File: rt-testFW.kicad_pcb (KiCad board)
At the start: 2 copper layers, 11 parts, among them J1 1Min, J2 2Min, J3 3Min, J4 5Min, SW1 TestStart-Peach, SW2 Reset-Black

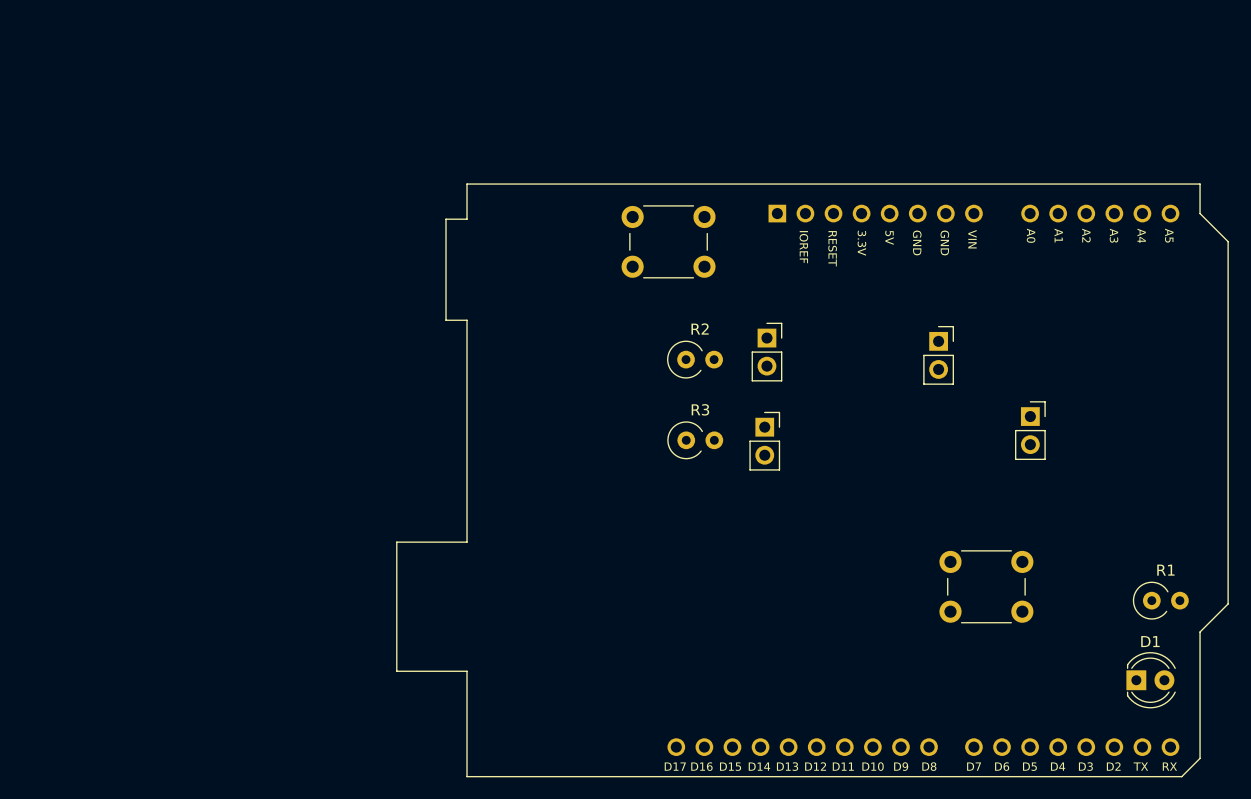
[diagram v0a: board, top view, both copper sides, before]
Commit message: initial iteration complete
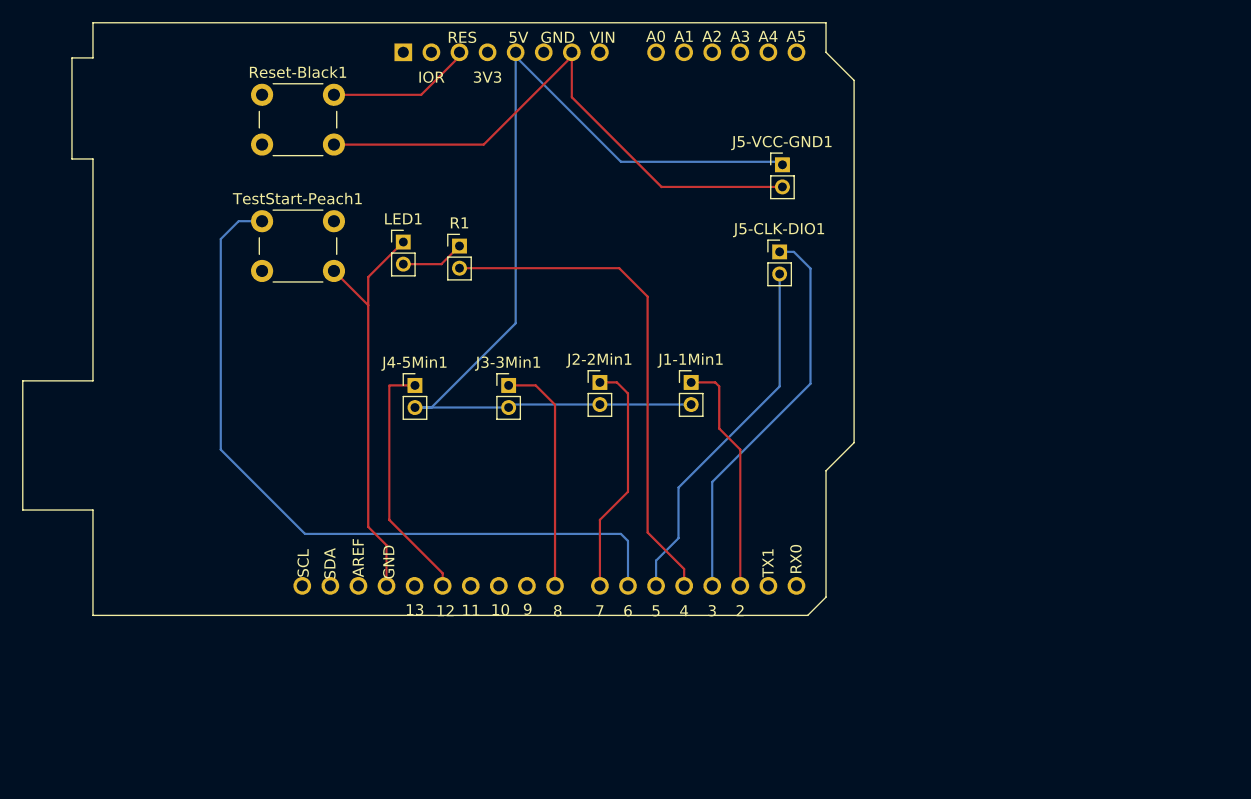
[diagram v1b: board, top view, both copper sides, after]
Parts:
- removed D1: LED, LED_THT:LED_D4.0mm
- removed J1: 1Min, Connector_PinSocket_2.54mm:PinSocket_1x02_P2.54mm_Vertical
- removed J2: 2Min, Connector_PinSocket_2.54mm:PinSocket_1x02_P2.54mm_Vertical
- removed J3: 3Min, Connector_PinSocket_2.54mm:PinSocket_1x02_P2.54mm_Vertical
- removed J4: 5Min, Connector_PinSocket_2.54mm:PinSocket_1x02_P2.54mm_Vertical
- removed R2, R3: R, Resistor_THT:R_Axial_DIN0309_L9.0mm_D3.2mm_P2.54mm_Vertical
- removed SW1: TestStart-Peach, Button_Switch_THT:SW_PUSH_6mm
- removed SW2: Reset-Black, Button_Switch_THT:SW_PUSH_6mm
- added J1-1Min1: Conn_01x02_Male, Connector_PinHeader_2.00mm:PinHeader_1x02_P2.00mm_Vertical, F.Cu at (220.3, 106.3)
- added J2-2Min1: Conn_01x02_Male, Connector_PinHeader_2.00mm:PinHeader_1x02_P2.00mm_Vertical, F.Cu at (212.1, 106.3)
- added J3-3Min1: Conn_01x02_Male, Connector_PinHeader_2.00mm:PinHeader_1x02_P2.00mm_Vertical, F.Cu at (203.8, 106.6)
- added J4-5Min1: Conn_01x02_Male, Connector_PinHeader_2.00mm:PinHeader_1x02_P2.00mm_Vertical, F.Cu at (195.4, 106.6)
- added J5-CLK-DIO1: Conn_01x02_Male, Connector_PinHeader_2.00mm:PinHeader_1x02_P2.00mm_Vertical, F.Cu at (228.3, 94.5)
- added J5-VCC-GND1: Conn_01x02_Male, Connector_PinHeader_2.00mm:PinHeader_1x02_P2.00mm_Vertical, F.Cu at (228.6, 86.6)
- added LED1: LED, Connector_PinHeader_2.00mm:PinHeader_1x02_P2.00mm_Vertical, F.Cu at (194.3, 93.6)
- added Reset-Black1: SW_Push_Dual, Button_Switch_THT:SW_PUSH_6mm, F.Cu at (181.5, 80.3)
- added TestStart-Peach1: SW_Push_Dual, Button_Switch_THT:SW_PUSH_6mm, F.Cu at (181.5, 91.7)
- R1: footprint Resistor_THT:R_Axial_DIN0309_L9.0mm_D3.2mm_P2.54mm_Vertical -> Connector_PinHeader_2.00mm:PinHeader_1x02_P2.00mm_Vertical
- moved R1 70.4 mm to (199.4, 94.0)
- moved A1 36.8 mm to (194.3, 76.5)
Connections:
- A1 pad 18: unconnected-(A1-D3-Pad18) -> Net-(A1-Pad18)
- A1 pad 20: unconnected-(A1-D5-Pad20) -> Net-(A1-Pad20)
- A1 pad 23: unconnected-(A1-D8-Pad23) -> Net-(A1-Pad23)
- A1 pad 27: unconnected-(A1-D12-Pad27) -> Net-(A1-Pad27)
- A1 pad 29: unconnected-(A1-GND-Pad29) -> Net-(A1-Pad29)
- A1 pad 7: unconnected-(A1-GND-Pad7) -> Net-(A1-Pad7)
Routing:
- net Net-(A1-Pad5): track 0.00 -> 89.7 mm
- net Net-(A1-Pad21): track 0.00 -> 68.1 mm
- net Net-(A1-Pad7): track 0.00 -> 51.3 mm
- net Net-(A1-Pad19): track 0.00 -> 45.6 mm
- net Net-(A1-Pad29): track 0.00 -> 37.9 mm
- net Net-(A1-Pad18): track 0.00 -> 36.2 mm
- net Net-(A1-Pad20): track 0.00 -> 33.2 mm
- net Net-(A1-Pad27): track 0.00 -> 22.7 mm
- net Net-(J1-1Min1-Pad1): track 0.00 -> 21.9 mm
- net Net-(A1-Pad22): track 0.00 -> 21.8 mm
- net Net-(A1-Pad23): track 0.00 -> 21.7 mm
- net Net-(A1-Pad3): track 0.00 -> 12.8 mm
- net Net-(R1-Pad1): track 0.00 -> 5.76 mm
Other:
- board text added: "10"
- board text added: "11"
- board text added: "12"
- board text added: "13"
- board text added: "2"
- board text added: "3"
- board text added: "3V3"
- board text added: "4"
- board text added: "5"
- board text added: "6"
- board text added: "7"
- board text added: "8"
- board text added: "9"
- board text added: "AREF"
- board text added: "IOR"
- board text added: "RES"
- board text added: "RX0"
- board text added: "SCL"
- board text added: "SDA"
- board text added: "TX1"
- board text removed: "3.3V"
- board text removed: "D10"
- board text removed: "D11"
- board text removed: "D12"
- board text removed: "D13"
- board text removed: "D14"
- board text removed: "D15"
- board text removed: "D16"
- board text removed: "D17"
- board text removed: "D2"
- board text removed: "D3"
- board text removed: "D4"
- board text removed: "D5"
- board text removed: "D6"
- board text removed: "D7"
- board text removed: "D8"
- board text removed: "D9"
- board text removed: "IOREF"
- board text removed: "RESET"
- board text removed: "RX"
- board text removed: "TX"
